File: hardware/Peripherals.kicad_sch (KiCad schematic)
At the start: 1 part, among them J6 USB_C_Receptacle_USB2.0_16P

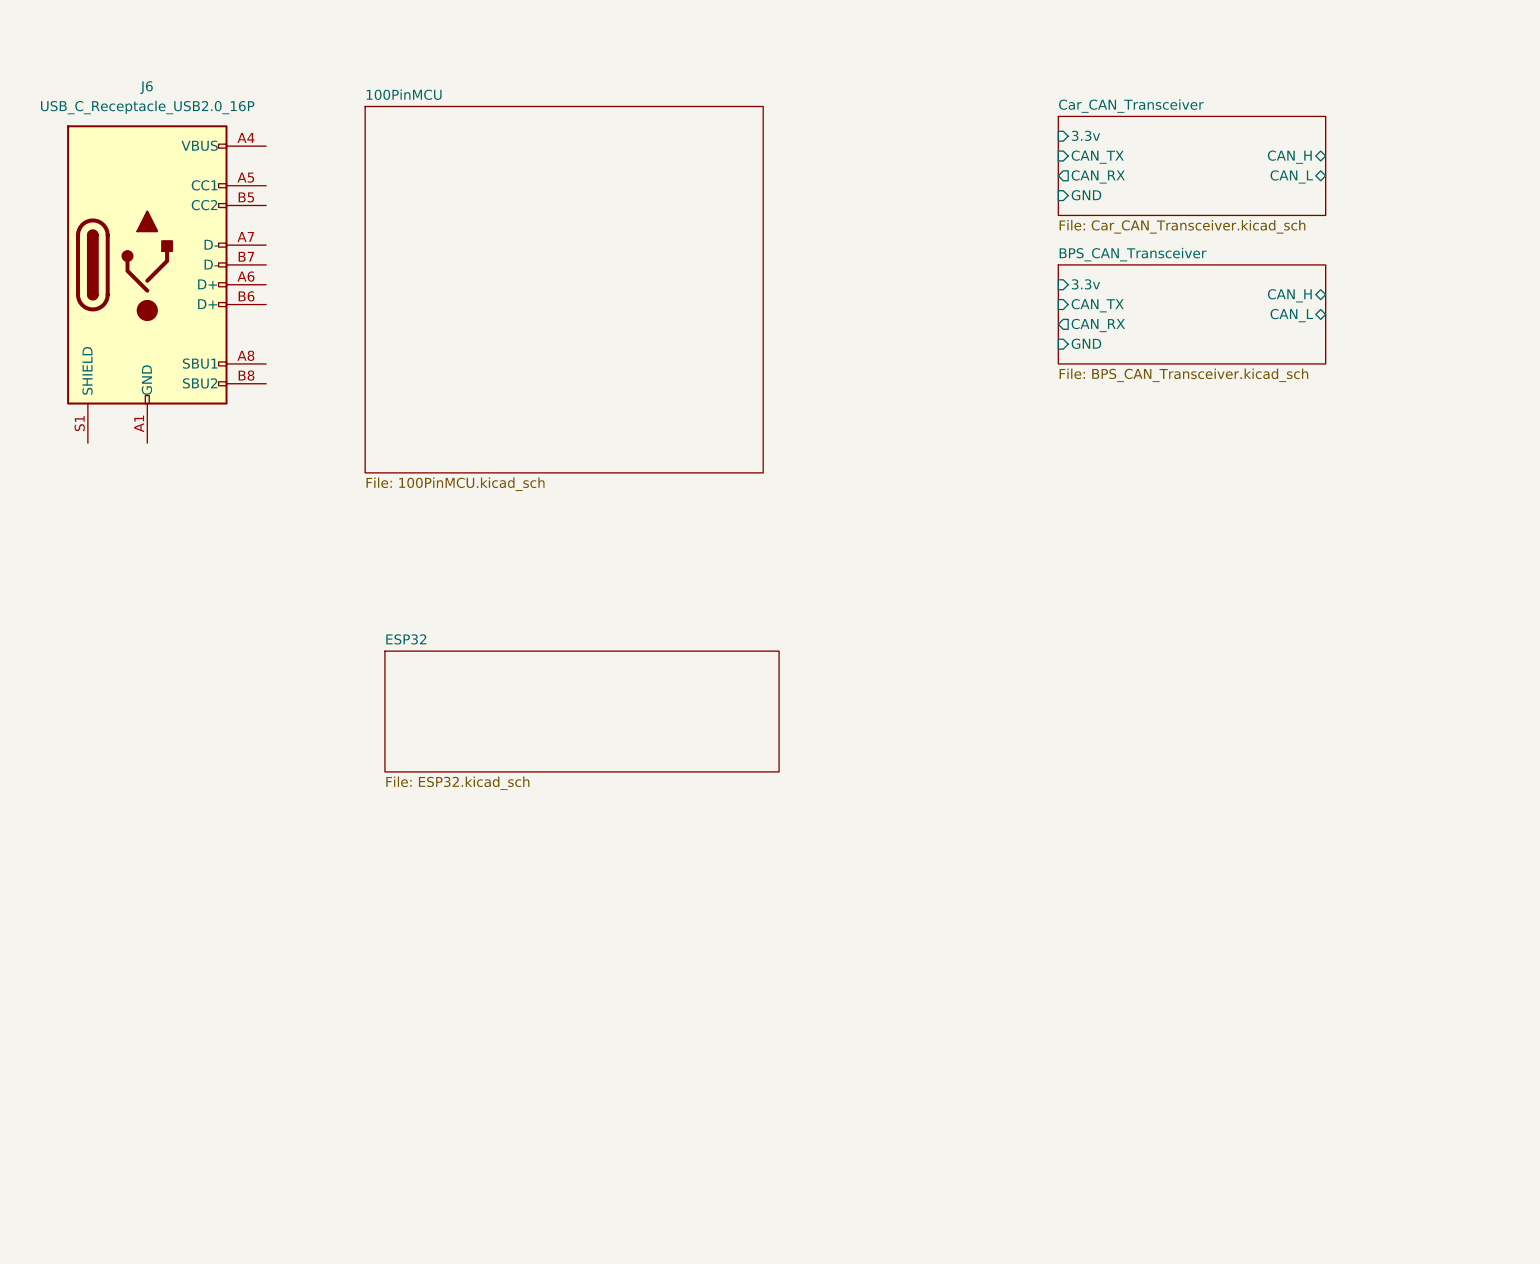
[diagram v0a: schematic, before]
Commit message: added more stuff wip
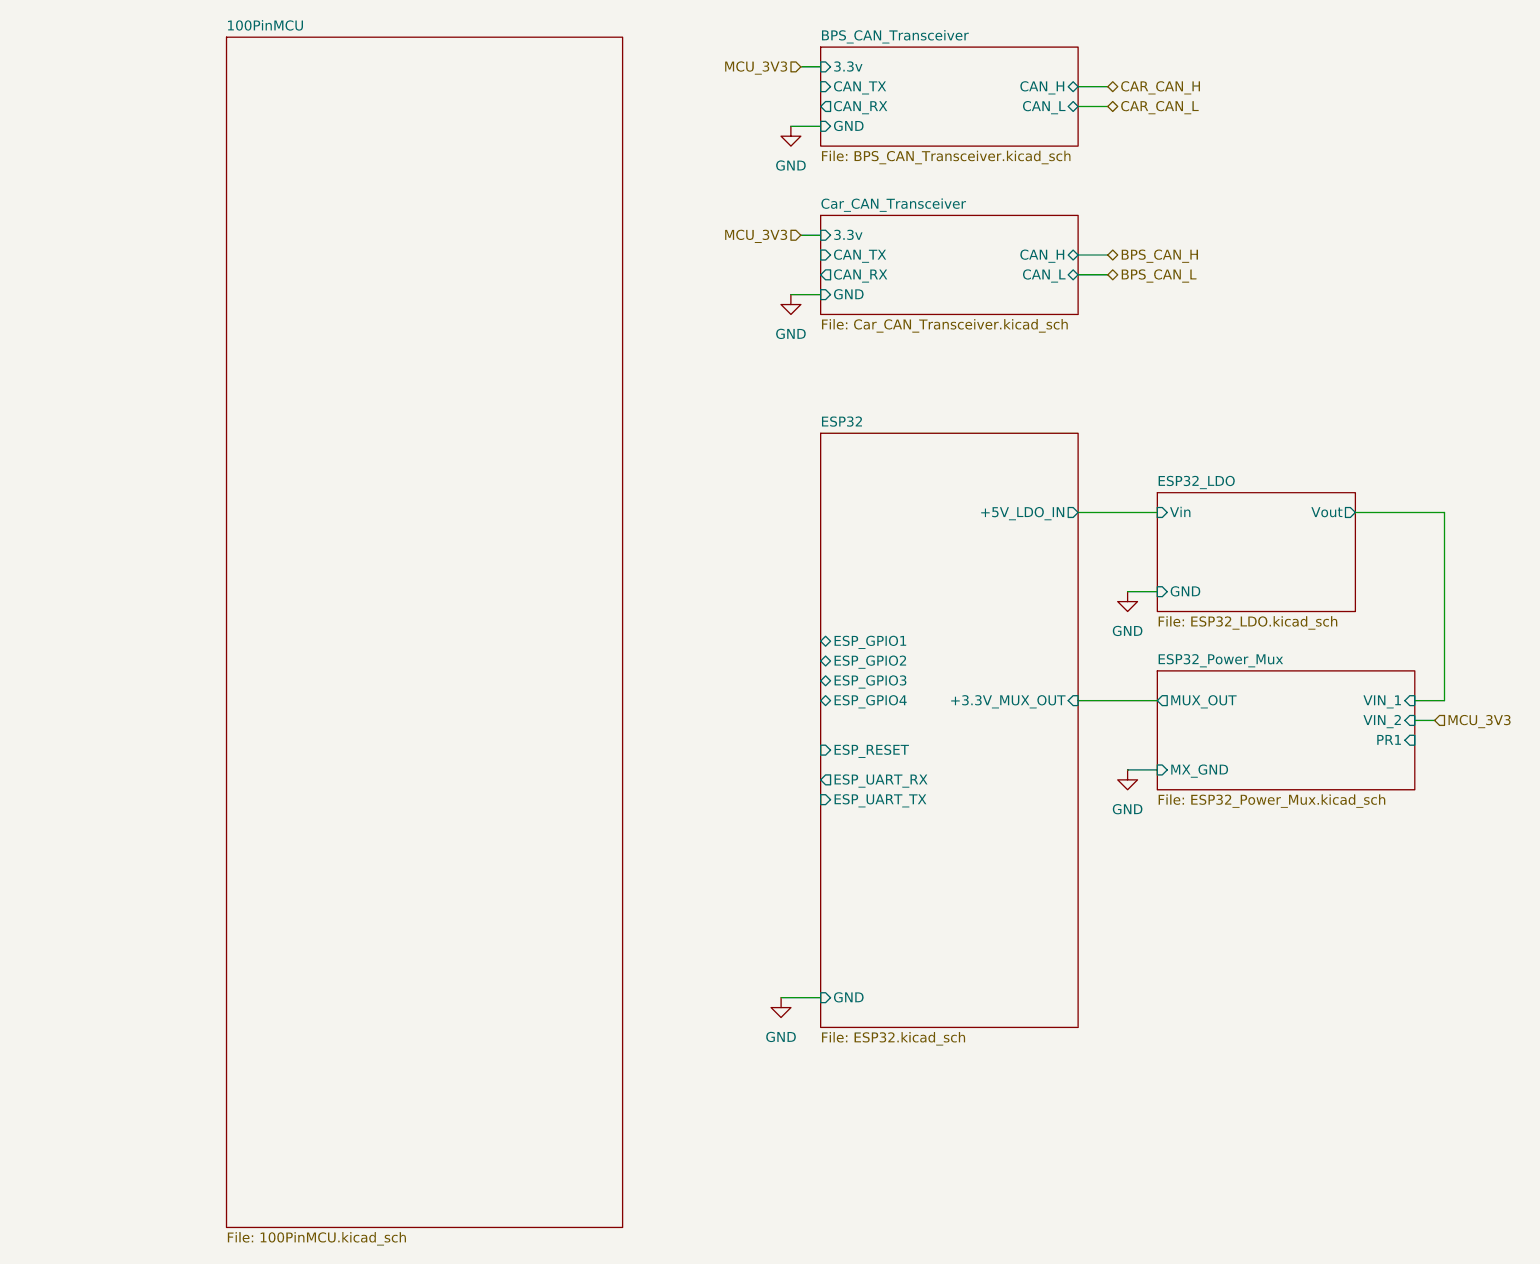
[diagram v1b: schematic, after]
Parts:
- removed J6: USB_C_Receptacle_USB2.0_16P, UTSVT_ICs:USB_C_Receptacle_GCT_USB4105-xx-A_16P_TopMnt_Horizontal, symbol utsvt_connectors:USB_C_Receptacle_USB2.0_16P
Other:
- added sheet ESP32_LDO (ESP32_LDO.kicad_sch)
- added sheet ESP32_Power_Mux (ESP32_Power_Mux.kicad_sch)
- sheet ESP32 ports: added +3.3V_MUX_OUT, +5V_LDO_IN, ESP_GPIO1, ESP_GPIO2, ESP_GPIO3, ESP_GPIO4, ESP_RESET, ESP_UART_RX, ESP_UART_TX, GND; removed none
